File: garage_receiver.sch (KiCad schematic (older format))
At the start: 11 parts, among them J1 Conn_01x04_Female, J2 Screw_Terminal_01x04, Q1 2N7002, SW1 SW_DIP_x08, U1 HT12D

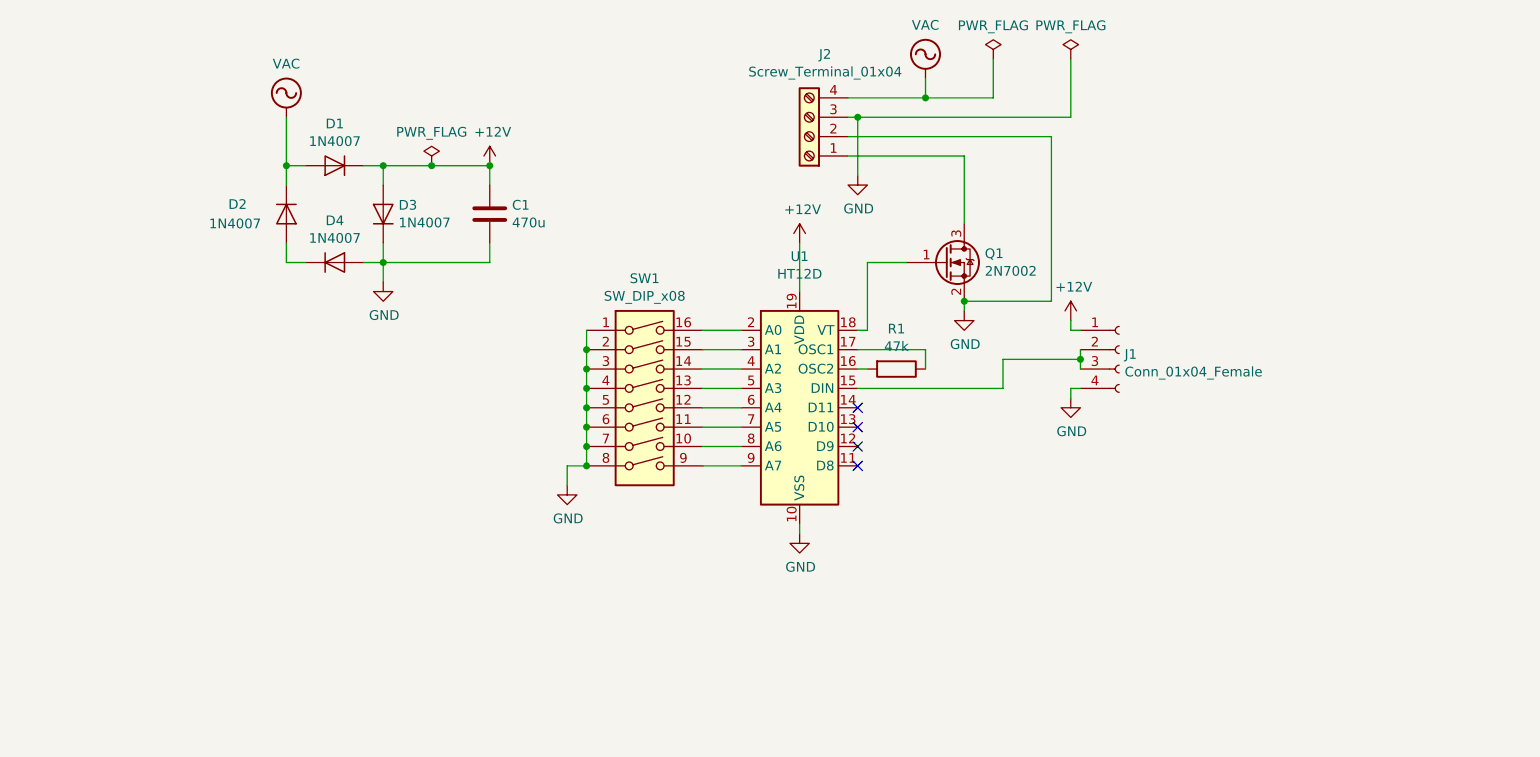
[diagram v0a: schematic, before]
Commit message: DC/DC Converter
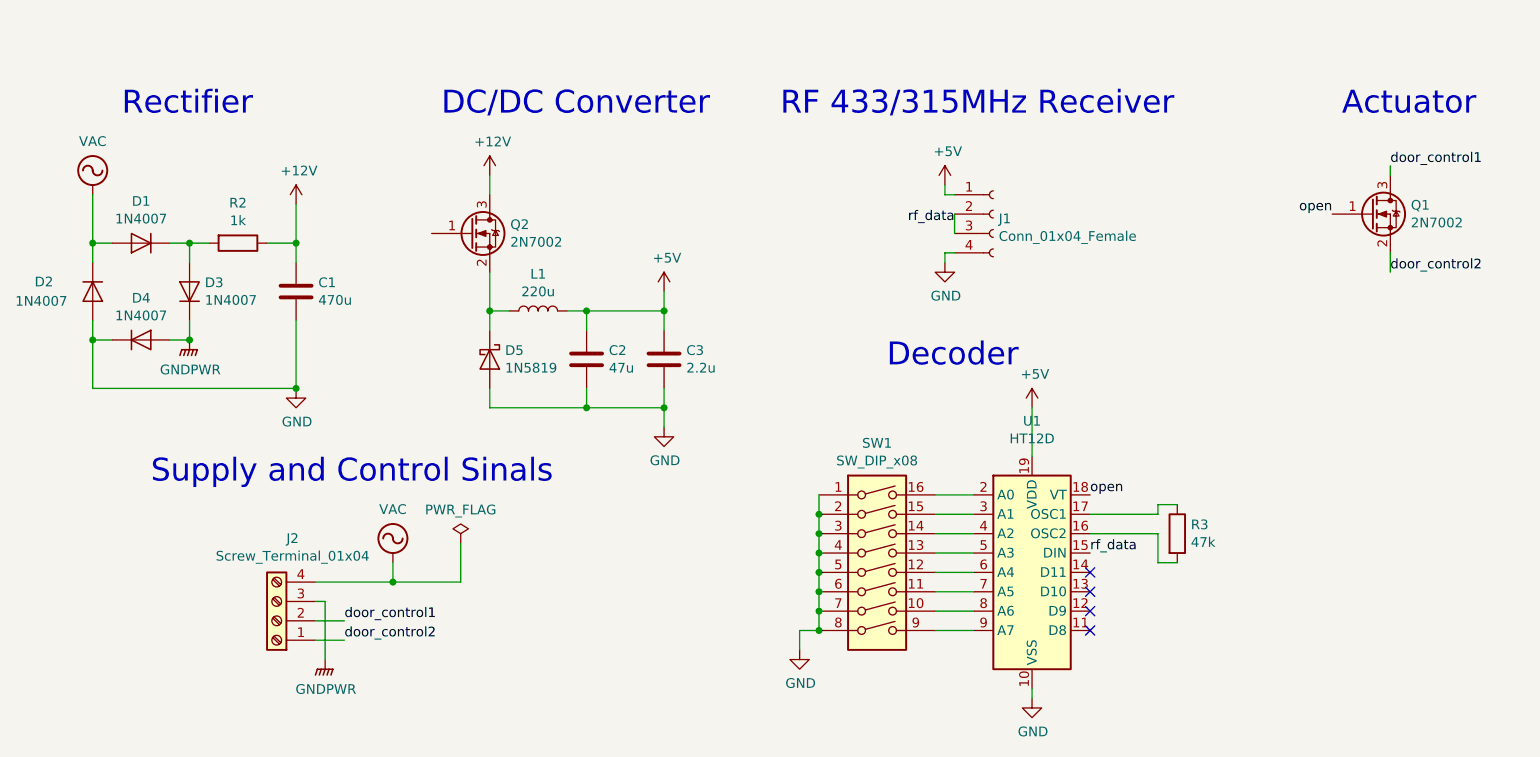
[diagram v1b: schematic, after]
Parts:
- removed R1: 47k, Resistor_SMD:R_0805_2012Metric, symbol Device:R
- added C2: 47u, Capacitor_THT:CP_Radial_D5.0mm_P2.00mm, symbol Device:C
- added C3: 2.2u, Capacitor_THT:C_Disc_D4.3mm_W1.9mm_P5.00mm, symbol Device:C
- added D5: 1N5819, Diode_THT:D_DO-41_SOD81_P10.16mm_Horizontal, symbol Diode:1N5819
- added L1: 220u, Inductor_SMD:L_10.4x10.4_H4.8, symbol Device:L
- added Q2: 2N7002, Package_TO_SOT_SMD:SOT-23, symbol Transistor_FET:2N7002
- added R2: 1k, Resistor_SMD:R_0805_2012Metric, symbol Device:R
- added R3: 47k, Resistor_SMD:R_0805_2012Metric, symbol Device:R
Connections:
- net +12V: now also Q2.3 (D), R2.1; no longer D1.1 (K), D3.2 (A), J1.1 (Pin_1), U1.19 (VDD)
- net GND: now also D2.2 (A), D4.1 (K), C2.2, C3.2, D5.2 (A); no longer D3.1 (K), D4.2 (A), J2.2 (Pin_2), J2.3 (Pin_3), Q1.2 (S)
- net rf_data: now reaches J1.2 (Pin_2), J1.3 (Pin_3), U1.15 (DIN)
- net at U1.16 (OSC2): now also R3.2
- net at U1.17 (OSC1): now also R3.1
- net open: now reaches Q1.1 (G), U1.18 (VT)
- net door_control1: now reaches Q1.3 (D)
- net door_control1: now also J2.2 (Pin_2); no longer J2.1 (Pin_1)
- new net: D1.1 (K), D3.2 (A), R2.2
- new net: D5.1 (K), L1.1, Q2.2 (S)
- new net +5V: C2.1, C3.1, J1.1 (Pin_1), L1.2, U1.19 (VDD)
- new net GNDPWR: D3.1 (K), D4.2 (A), J2.3 (Pin_3)
- new net door_control2: J2.1 (Pin_1), Q1.2 (S)
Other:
- note added: "Actuator"
- note added: "DC/DC Converter"
- note added: "Decoder"
- note added: "RF 433/315MHz Receiver"
- note added: "Rectifier"
- note added: "Supply and Control Sinals"
- moved on the sheet: C1, D1, D2, D3, D4, J1, J2, Q1, SW1, U1

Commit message: DC/DC Converter Controller
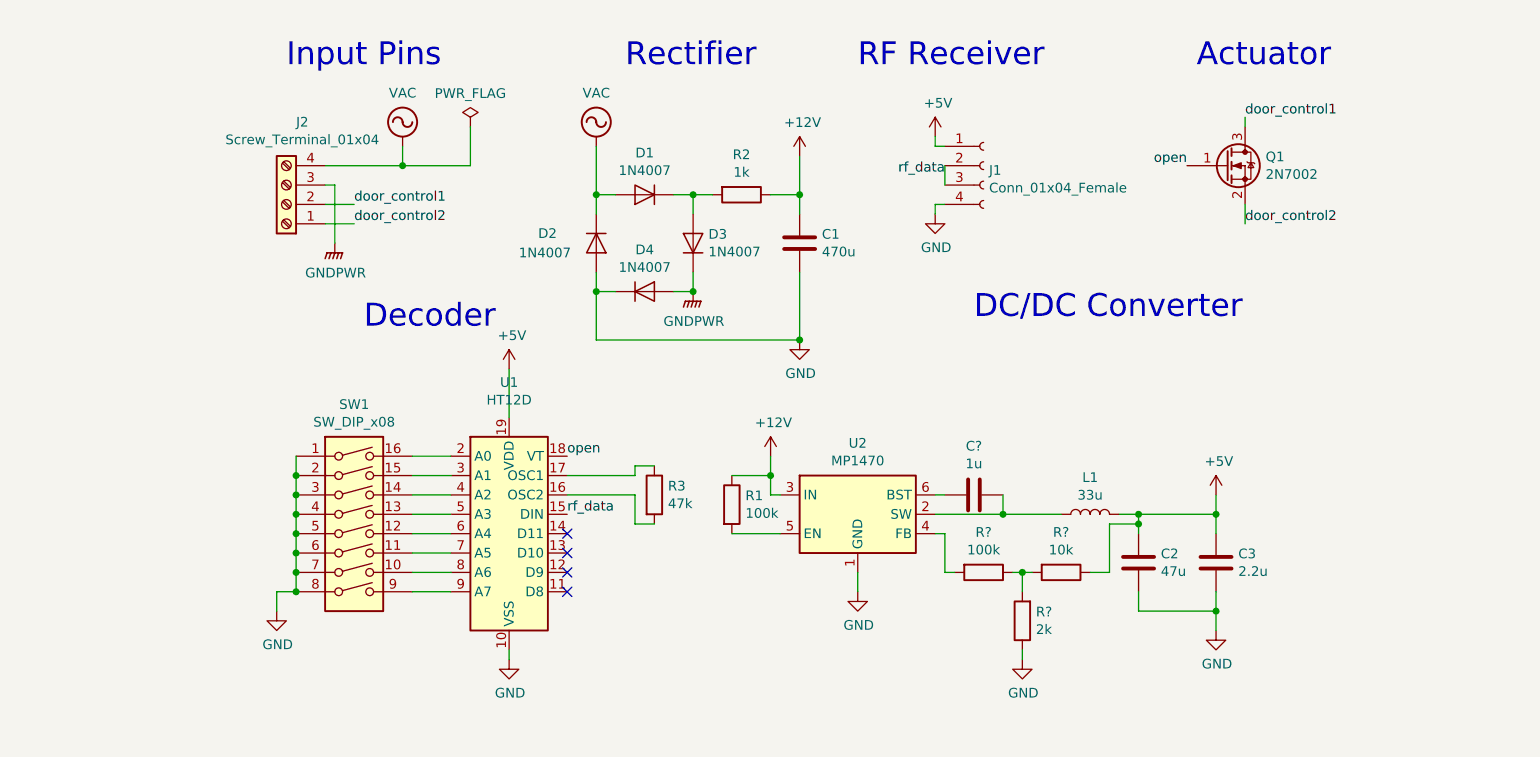
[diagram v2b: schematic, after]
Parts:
- removed D5: 1N5819, Diode_THT:D_DO-41_SOD81_P10.16mm_Horizontal, symbol Diode:1N5819
- removed Q2: 2N7002, Package_TO_SOT_SMD:SOT-23, symbol Transistor_FET:2N7002
- added C?: 1u, Capacitor_THT:CP_Radial_D4.0mm_P1.50mm, symbol Device:C
- added R1, R?: 100k, symbol Device:R
- added R?: 10k, symbol Device:R
- added R?: 2k, symbol Device:R
- added U2: MP1470, Package_TO_SOT_SMD:TSOT-23-6, symbol Regulator_Switching:MP1470
- L1: value 220u -> 33u
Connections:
- net +12V: now also R1.1, U2.3 (IN)
- net +5V: now also R?.1
- net GND: now also R?.1, U2.1 (GND)
- net at L1.1: now also C?.1, U2.2 (SW)
- new net: R?.2, U2.4 (FB)
- new net: R1.2, U2.5 (EN)
- new net: C?.2, U2.6 (BST)
- new net: R?.1, R?.2, R?.2
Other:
- note added: "Input Pins"
- note added: "RF Receiver"
- note removed: "RF 433/315MHz Receiver"
- note removed: "Supply and Control Sinals"
- moved on the sheet: C1, C2, C3, D1, D2, D3, D4, J1, J2, L1, Q1, R2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
